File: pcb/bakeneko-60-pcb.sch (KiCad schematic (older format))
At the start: 18 parts, among them J1 JST SH 4-pin, J2 AVR-ISP-6, SW1 Reset, U1 USBLC6-2SC6, U2 ATmega32U4-AU, Y1 16MHz

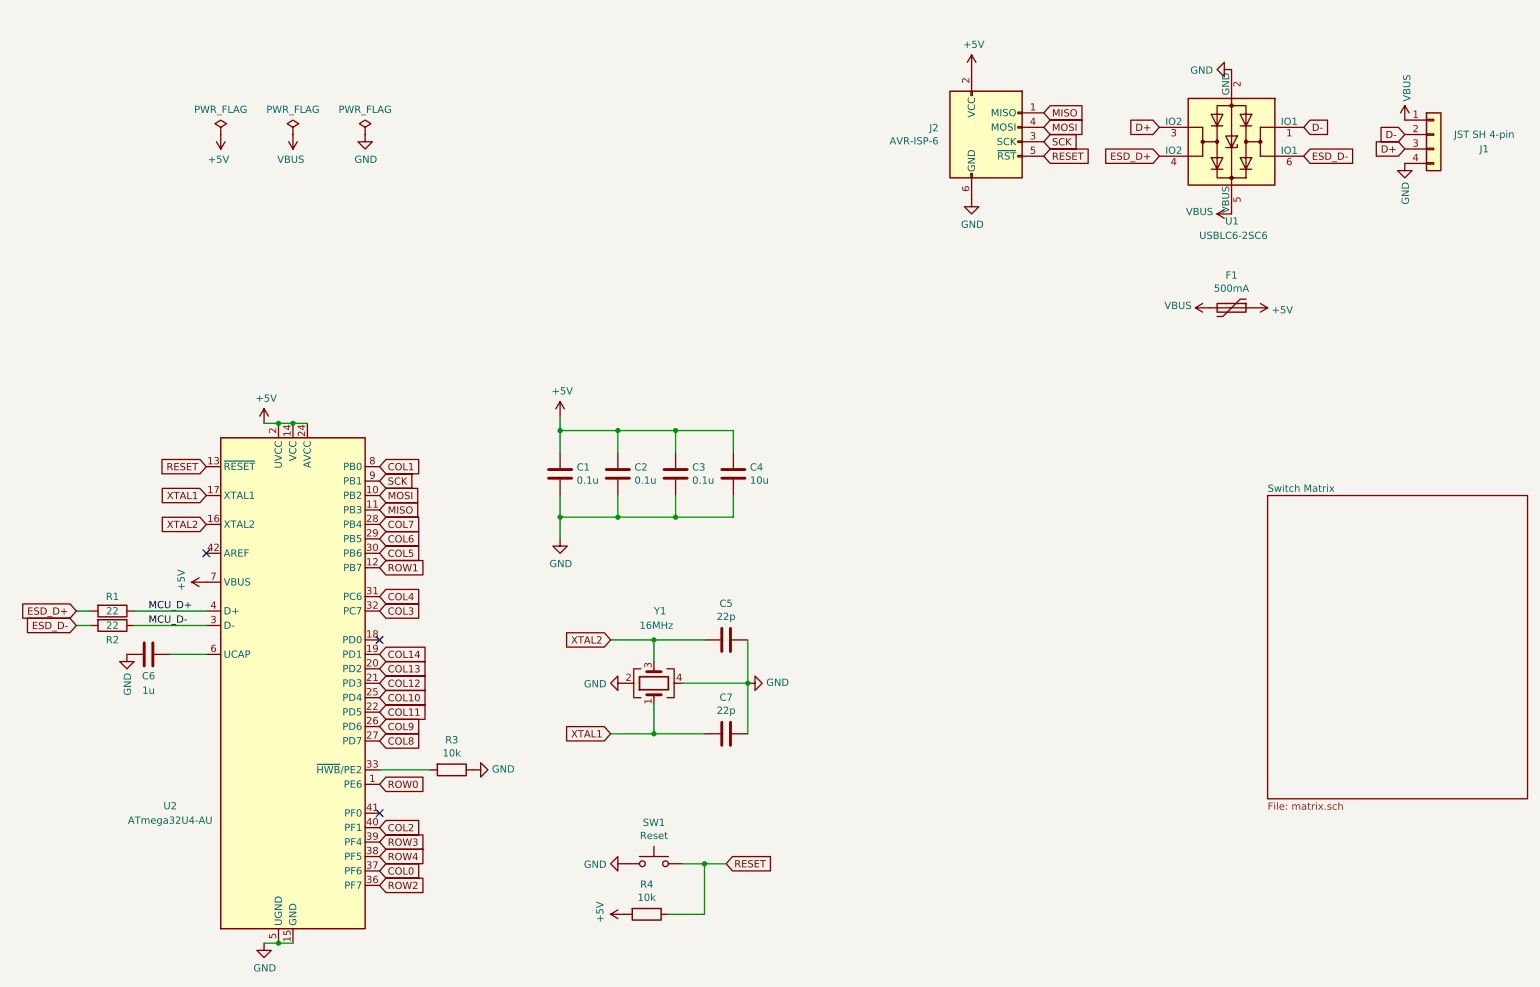
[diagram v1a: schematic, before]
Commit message: Update PCB
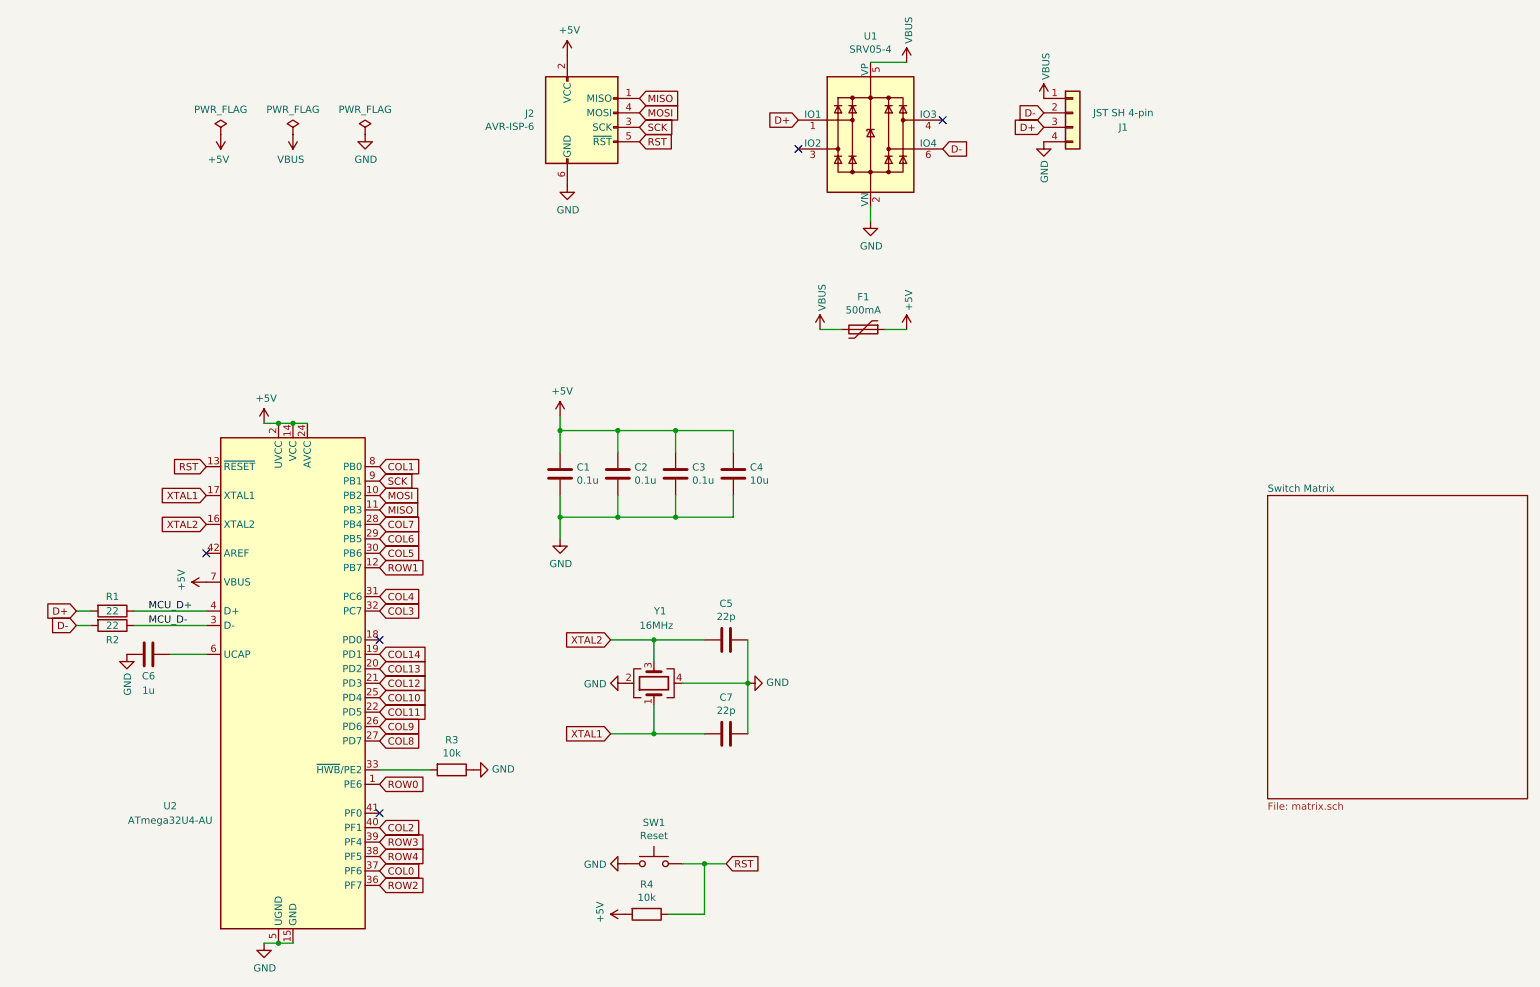
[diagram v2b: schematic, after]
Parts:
- removed U1: USBLC6-2SC6, Package_TO_SOT_SMD:SOT-23-6, symbol Power_Protection:USBLC6-2SC6
- added U1: SRV05-4, Package_TO_SOT_SMD:SOT-23-6, symbol Power_Protection:SRV05-4
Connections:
- net ESD_D+ is gone; now on net D+: R1.2
- net ESD_D- is gone; now on net D-: R2.2
- net D+: now also U1.1 (IO1)
- net D-: now also U1.6 (IO4)
- net GND: now also U1.2 (VN)
- net VBUS: now also U1.5 (VP)
- net RESET renamed RST
- no-connect marks 3 -> 5
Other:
- moved on the sheet: F1, J1, J2
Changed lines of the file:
@@
 encoding utf-8
 Sheet 1 2
-Title "Bakeneko 65"
+Title "Bakeneko 60 V3"
 Date "2020-08-01"
 Rev "1"
@@
 L Device:Polyfuse F1
 U 1 1 5F2505EB
-P 8850 2800
-F 0 "F1" V 8625 2800 50  0000 C CNN
-F 1 "500mA" V 8716 2800 50  0000 C CNN
-F 2 "Fuse:Fuse_1206_3216Metric" H 8900 2600 50  0001 L CNN
-F 3 "~" H 8850 2800 50  0001 C CNN
-F 4 "C70076" H 8850 2800 50  0001 C CNN "LCSC Part #"
-	1    8850 2800
+P 6300 2950
+F 0 "F1" V 6075 2950 50  0000 C CNN
+F 1 "500mA" V 6166 2950 50  0000 C CNN
+F 2 "Fuse:Fuse_1206_3216Metric" H 6350 2750 50  0001 L CNN
+F 3 "~" H 6300 2950 50  0001 C CNN
+F 4 "C70076" H 6300 2950 50  0001 C CNN "LCSC Part #"
+	1    6300 2950
 	0    1    1    0
 $EndComp
@@
 L Connector_Generic:Conn_01x04 J1
 U 1 1 5F252816
-P 10250 1600
-F 0 "J1" H 10600 1500 50  0000 C CNN
-F 1 "JST SH 4-pin" H 10600 1600 50  0000 C CNN
-F 2 "Connector_JST:JST_SH_SM04B-SRSS-TB_1x04-1MP_P1.00mm_Horizontal" H 10250 1600 50  0001 C CNN
-F 3 "~" H 10250 1600 50  0001 C CNN
-F 4 "C160404" H 10250 1600 50  0001 C CNN "LCSC Part #"
-	1    10250 1600
-	1    0    0    -1
-$EndComp
-$Comp
-L power:GND #PWR02
-U 1 1 5F256D2D
-P 8850 1150
-F 0 "#PWR02" H 8850 900 50  0001 C CNN
-F 1 "GND" V 8855 1022 50  0000 R CNN
-F 2 "" H 8850 1150 50  0001 C CNN
-F 3 "" H 8850 1150 50  0001 C CNN
-	1    8850 1150
-	0    1    1    0
+P 7750 1450
+F 0 "J1" H 8100 1350 50  0000 C CNN
+F 1 "JST SH 4-pin" H 8100 1450 50  0000 C CNN
+F 2 "Connector_JST:JST_SH_SM04B-SRSS-TB_1x04-1MP_P1.00mm_Horizontal" H 7750 1450 50  0001 C CNN
+F 3 "~" H 7750 1450 50  0001 C CNN
+F 4 "C160404" H 7750 1450 50  0001 C CNN "LCSC Part #"
+	1    7750 1450
+	1    0    0    -1
 $EndComp
 $Comp
@@
 	0    1    1    0
 $EndComp
-Text GLabel 10050 1600 0    50   Input ~ 0
+Text GLabel 7550 1450 0    50   Input ~ 0
 D-
-Text GLabel 10050 1700 0    50   Input ~ 0
+Text GLabel 7550 1550 0    50   Input ~ 0
 D+
 $Comp
@@
 L power:VBUS #PWR03
 U 1 1 5F275D18
-P 10050 1500
-F 0 "#PWR03" H 10050 1350 50  0001 C CNN
-F 1 "VBUS" V 10065 1628 50  0000 L CNN
-F 2 "" H 10050 1500 50  0001 C CNN
-F 3 "" H 10050 1500 50  0001 C CNN
-	1    10050 1500
+P 7550 1350
+F 0 "#PWR03" H 7550 1200 50  0001 C CNN
+F 1 "VBUS" V 7565 1478 50  0000 L CNN
+F 2 "" H 7550 1350 50  0001 C CNN
+F 3 "" H 7550 1350 50  0001 C CNN
+	1    7550 1350
 	1    0    0    -1
 $EndComp
@@
 $EndComp
 $Comp
-L power:VBUS #PWR09
-U 1 1 5F276E32
-P 8850 2150
-F 0 "#PWR09" H 8850 2000 50  0001 C CNN
-F 1 "VBUS" V 8865 2278 50  0000 L CNN
-F 2 "" H 8850 2150 50  0001 C CNN
-F 3 "" H 8850 2150 50  0001 C CNN
-	1    8850 2150
-	0    -1   -1   0
-$EndComp
-$Comp
 L power:VBUS #PWR010
 U 1 1 5F277A1C
-P 8700 2800
-F 0 "#PWR010" H 8700 2650 50  0001 C CNN
-F 1 "VBUS" V 8715 2927 50  0000 L CNN
-F 2 "" H 8700 2800 50  0001 C CNN
-F 3 "" H 8700 2800 50  0001 C CNN
-	1    8700 2800
-	0    -1   -1   0
-$EndComp
-Text GLabel 8350 1550 0    50   Input ~ 0
-D+
-Text GLabel 9350 1550 2    50   Input ~ 0
-D-
+P 6000 2950
+F 0 "#PWR010" H 6000 2800 50  0001 C CNN
+F 1 "VBUS" V 6015 3077 50  0000 L CNN
+F 2 "" H 6000 2950 50  0001 C CNN
+F 3 "" H 6000 2950 50  0001 C CNN
+	1    6000 2950
+	1    0    0    -1
+$EndComp
 $Comp
 L Switch:SW_Push SW1
@@
 	0    1    1    0
 $EndComp
-Text GLabel 5350 6650 2    50   Input ~ 0
-RESET
 $Comp
 L Device:R R4
@@
 	5200 6650 5350 6650
 Text GLabel 1750 3900 0    50   Input ~ 0
-RESET
+RST
 Text GLabel 1750 4100 0    50   Input ~ 0
 XTAL1
@@
 L Connector:AVR-ISP-6 J2
 U 1 1 5F4C9CCE
-P 7150 1650
-F 0 "J2" H 6821 1746 50  0000 R CNN
-F 1 "AVR-ISP-6" H 6821 1655 50  0000 R CNN
-F 2 "random-keyboard-parts:Reset_Pretty" V 6900 1700 50  0001 C CNN
-F 3 " ~" H 5875 1100 50  0001 C CNN
-	1    7150 1650
+P 4350 1550
+F 0 "J2" H 4021 1646 50  0000 R CNN
+F 1 "AVR-ISP-6" H 4021 1555 50  0000 R CNN
+F 2 "random-keyboard-parts:Reset_Pretty" V 4100 1600 50  0001 C CNN
+F 3 " ~" H 3075 1000 50  0001 C CNN
+	1    4350 1550
 	1    0    0    -1
 $EndComp
@@
 L power:GND #PWR08
 U 1 1 5F4D2BF6
-P 7050 2050
-F 0 "#PWR08" H 7050 1800 50  0001 C CNN
-F 1 "GND" H 7055 1877 50  0000 C CNN
-F 2 "" H 7050 2050 50  0001 C CNN
-F 3 "" H 7050 2050 50  0001 C CNN
-	1    7050 2050
-	1    0    0    -1
-$EndComp
-Text GLabel 7550 1450 2    50   Input ~ 0
+P 4250 1950
+F 0 "#PWR08" H 4250 1700 50  0001 C CNN
+F 1 "GND" H 4255 1777 50  0000 C CNN
+F 2 "" H 4250 1950 50  0001 C CNN
+F 3 "" H 4250 1950 50  0001 C CNN
+	1    4250 1950
+	1    0    0    -1
+$EndComp
+Text GLabel 4750 1350 2    50   Input ~ 0
 MISO
-Text GLabel 7550 1550 2    50   Input ~ 0
+Text GLabel 4750 1450 2    50   Input ~ 0
 MOSI
-Text GLabel 7550 1650 2    50   Input ~ 0
+Text GLabel 4750 1550 2    50   Input ~ 0
 SCK
-Text GLabel 7550 1750 2    50   Input ~ 0
-RESET
+Text GLabel 4750 1650 2    50   Input ~ 0
+RST
 Text GLabel 2950 4200 2    50   Input ~ 0
 MISO
@@
 Text GLabel 2950 6800 2    50   Input ~ 0
 ROW2
-$Comp
-L Power_Protection:USBLC6-2SC6 U1
-U 1 1 5F25444E
-P 8850 1650
-F 0 "U1" H 8800 2200 50  0000 L CNN
-F 1 "USBLC6-2SC6" H 8600 2300 50  0000 L CNN
-F 2 "Package_TO_SOT_SMD:SOT-23-6" H 8850 1150 50  0001 C CNN
-F 3 "https://www.st.com/resource/en/datasheet/usblc6-2.pdf" H 9050 2000 50  0001 C CNN
-F 4 "C7519" H 8850 1650 50  0001 C CNN "LCSC Part #"
-	1    8850 1650
-	-1   0    0    1
-$EndComp
 Text GLabel 2950 6100 2    50   Input ~ 0
 ROW0
@@
 L power:GND #PWR07
 U 1 1 5F253A4B
-P 10050 1800
-F 0 "#PWR07" H 10050 1550 50  0001 C CNN
-F 1 "GND" V 10055 1672 50  0000 R CNN
-F 2 "" H 10050 1800 50  0001 C CNN
-F 3 "" H 10050 1800 50  0001 C CNN
-	1    10050 1800
-	1    0    0    -1
-$EndComp
-Text GLabel 850  5000 0    50   Input ~ 0
-ESD_D-
+P 7550 1650
+F 0 "#PWR07" H 7550 1400 50  0001 C CNN
+F 1 "GND" V 7555 1522 50  0000 R CNN
+F 2 "" H 7550 1650 50  0001 C CNN
+F 3 "" H 7550 1650 50  0001 C CNN
+	1    7550 1650
+	1    0    0    -1
+$EndComp
 Wire Wire Line
 	850  5000 950  5000
-Text GLabel 850  4900 0    50   Input ~ 0
-ESD_D+
 Wire Wire Line
 	850  4900 950  4900
-Text GLabel 9350 1750 2    50   Input ~ 0
-ESD_D-
-Text GLabel 8350 1750 0    50   Input ~ 0
-ESD_D+
 $Comp
 L power:+5V #PWR04
@@
 L power:+5V #PWR011
 U 1 1 5F3C7287
-P 9000 2800
-F 0 "#PWR011" H 9000 2650 50  0001 C CNN
-F 1 "+5V" V 9015 2928 50  0000 L CNN
-F 2 "" H 9000 2800 50  0001 C CNN
-F 3 "" H 9000 2800 50  0001 C CNN
-	1    9000 2800
-	0    1    1    0
+P 6600 2950
+F 0 "#PWR011" H 6600 2800 50  0001 C CNN
+F 1 "+5V" V 6615 3078 50  0000 L CNN
+F 2 "" H 6600 2950 50  0001 C CNN
+F 3 "" H 6600 2950 50  0001 C CNN
+	1    6600 2950
+	1    0    0    -1
 $EndComp
 $Comp
 L power:+5V #PWR01
 U 1 1 5F3D1A13
-P 7050 1150
-F 0 "#PWR01" H 7050 1000 50  0001 C CNN
-F 1 "+5V" H 7065 1323 50  0000 C CNN
-F 2 "" H 7050 1150 50  0001 C CNN
-F 3 "" H 7050 1150 50  0001 C CNN
-	1    7050 1150
+P 4250 1050
+F 0 "#PWR01" H 4250 900 50  0001 C CNN
+F 1 "+5V" H 4265 1223 50  0000 C CNN
+F 2 "" H 4250 1050 50  0001 C CNN
+F 3 "" H 4250 1050 50  0001 C CNN
+	1    4250 1050
 	1    0    0    -1
 $EndComp
@@
 ROW3
 NoConn ~ 2950 5100
+$Comp
+L Power_Protection:SRV05-4 U1
+U 1 1 60AFA3F3
+P 6350 1600
+F 0 "U1" H 6350 2281 50  0000 C CNN
+F 1 "SRV05-4" H 6350 2190 50  0000 C CNN
+F 2 "Package_TO_SOT_SMD:SOT-23-6" H 7050 1150 50  0001 C CNN
+F 3 "http://www.onsemi.com/pub/Collateral/SRV05-4-D.PDF" H 6350 1600 50  0001 C CNN
+F 4 "C85364" H 6350 1600 50  0001 C CNN "LCSC Part #"
+	1    6350 1600
+	1    0    0    -1
+$EndComp
+$Comp
+L power:GND #PWR0101
+U 1 1 60AFD50E
+P 6350 2200
+F 0 "#PWR0101" H 6350 1950 50  0001 C CNN
+F 1 "GND" H 6355 2027 50  0000 C CNN
+F 2 "" H 6350 2200 50  0001 C CNN
+F 3 "" H 6350 2200 50  0001 C CNN
+	1    6350 2200
+	1    0    0    -1
+$EndComp
+$Comp
+L power:VBUS #PWR0102
+U 1 1 60B00B85
+P 6600 1100
+F 0 "#PWR0102" H 6600 950 50  0001 C CNN
+F 1 "VBUS" V 6615 1228 50  0000 L CNN
+F 2 "" H 6600 1100 50  0001 C CNN
+F 3 "" H 6600 1100 50  0001 C CNN
+	1    6600 1100
+	1    0    0    -1
+$EndComp
+Text GLabel 6850 1700 2    50   Input ~ 0
+D-
+Text GLabel 5850 1500 0    50   Input ~ 0
+D+
+Wire Wire Line
+	6350 2100 6350 2200
+Wire Wire Line
+	6600 1100 6350 1100
+Wire Wire Line
+	6600 2950 6450 2950
+Wire Wire Line
+	6000 2950 6150 2950
+Text GLabel 5350 6650 2    50   Input ~ 0
+RST
+Text GLabel 850  4900 0    50   Input ~ 0
+D+
+Text GLabel 850  5000 0    50   Input ~ 0
+D-
+NoConn ~ 6850 1500
+NoConn ~ 5850 1700
 $EndSCHEMATC
